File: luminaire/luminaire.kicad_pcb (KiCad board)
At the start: 2 copper layers, 18 x 78 mm, 19 parts, among them Q1 FMMT618, SW1 SW_DP3T, U1 zxsc310

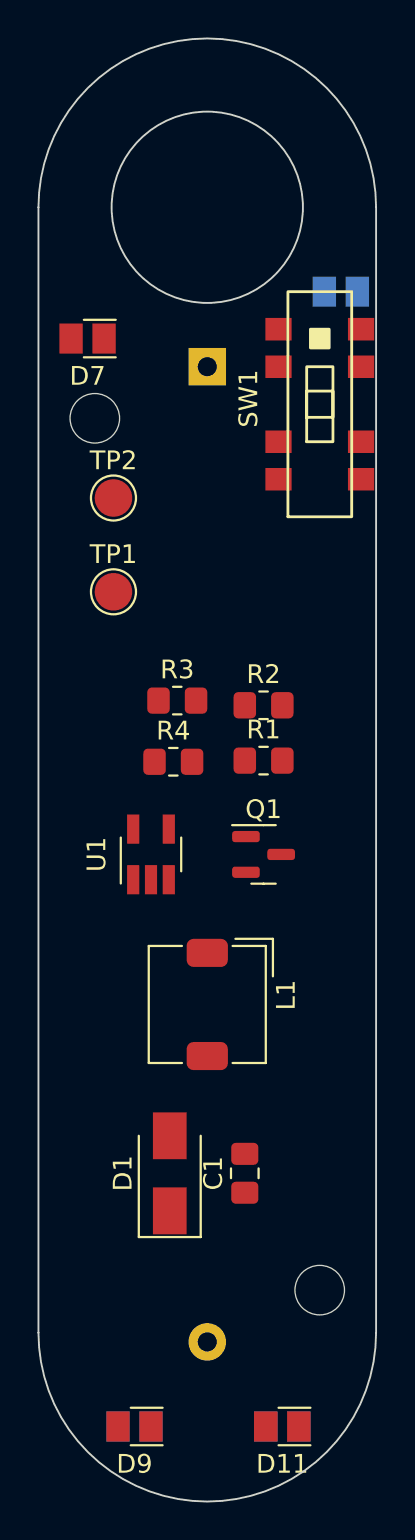
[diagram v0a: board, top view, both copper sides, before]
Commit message: Finalise design
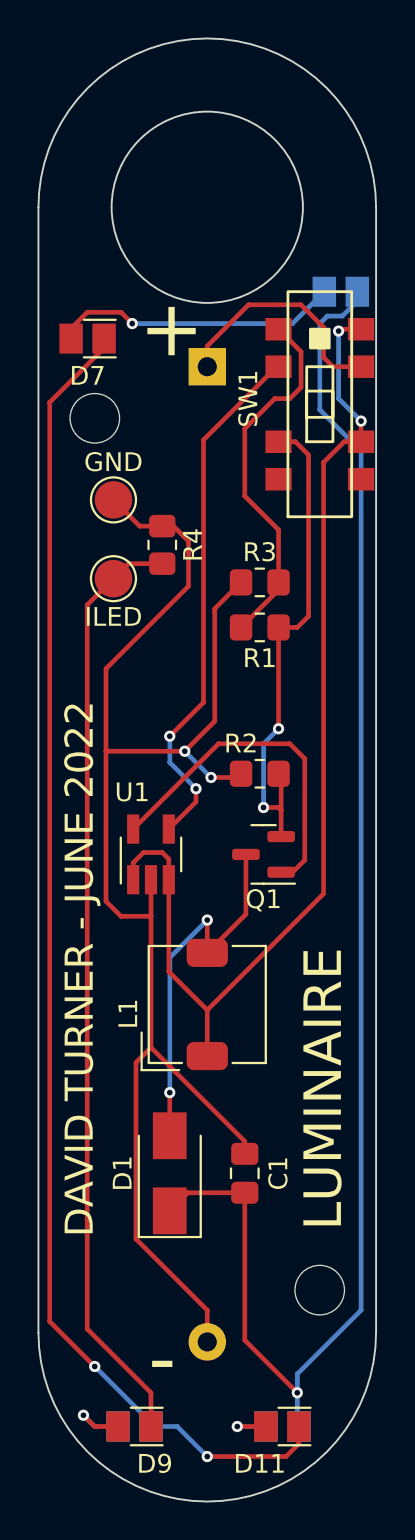
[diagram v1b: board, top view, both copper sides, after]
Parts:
- moved R4 11.6 mm to (147.6, 64.0), turned to -90 degrees
- moved R3 7.68 mm to (152.8, 66.0), turned to 180 degrees
- moved R1 7.10 mm to (152.8, 68.4), turned to 180 degrees
- moved TP1 4.90 mm to (145.0, 61.6)
- moved TP2 4.30 mm to (145.0, 65.8)
- moved R2 3.66 mm to (152.8, 76.2), turned to 180 degrees
- turned L1 to 90 degrees
- turned Q1 to 180 degrees
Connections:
- D6 pad 1: Net-(D10-Pad1) -> Net-(D6-Pad1)
- D7 pad 2: Net-(D10-Pad1) -> Net-(D6-Pad1)
- U1 pad 3: Net-(BT1-Pad2) -> Net-(L1-Pad1)
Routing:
- net Net-(BT1-Pad2): track 0.00 -> 81.0 mm, vias 0 -> 2
- net Net-(C1-Pad1): track 0.00 -> 80.4 mm, vias 0 -> 1
- net Net-(D11-Pad1): track 0.00 -> 71.2 mm, vias 0 -> 2
- net Net-(L1-Pad1): track 0.00 -> 56.4 mm, vias 0 -> 2
- net Net-(D9-Pad1): track 0.00 -> 50.1 mm
- net Net-(SW1-Pad7): track 0.00 -> 28.3 mm, vias 0 -> 2
- net Net-(Q1-Pad2): track 0.00 -> 26.7 mm, vias 0 -> 2
- net Net-(D1-Pad2): track 0.00 -> 20.2 mm, vias 0 -> 2
- net Net-(R1-Pad2): track 0.00 -> 19.7 mm
- net Net-(Q1-Pad1): track 0.00 -> 18.3 mm
- net Net-(D6-Pad1): track 0.00 -> 15.3 mm, vias 0 -> 1
- net Net-(BT1-Pad1): track 0.00 -> 12.5 mm
- net Net-(D8-Pad1): track 0.00 -> 4.18 mm, vias 0 -> 1
- net Net-(D10-Pad1): track 0.00 -> 3.04 mm, vias 0 -> 1
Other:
- board text added: "DAVID TURNER - JUNE 2022"
- board text added: "LUMINAIRE"
